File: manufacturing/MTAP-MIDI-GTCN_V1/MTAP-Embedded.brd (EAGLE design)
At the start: 160 x 100 mm, 32 parts, among them IC1 ESP32-WROOM-32D, IC2 AMS1117-3.3, X1 USB4140-GF-0230-C

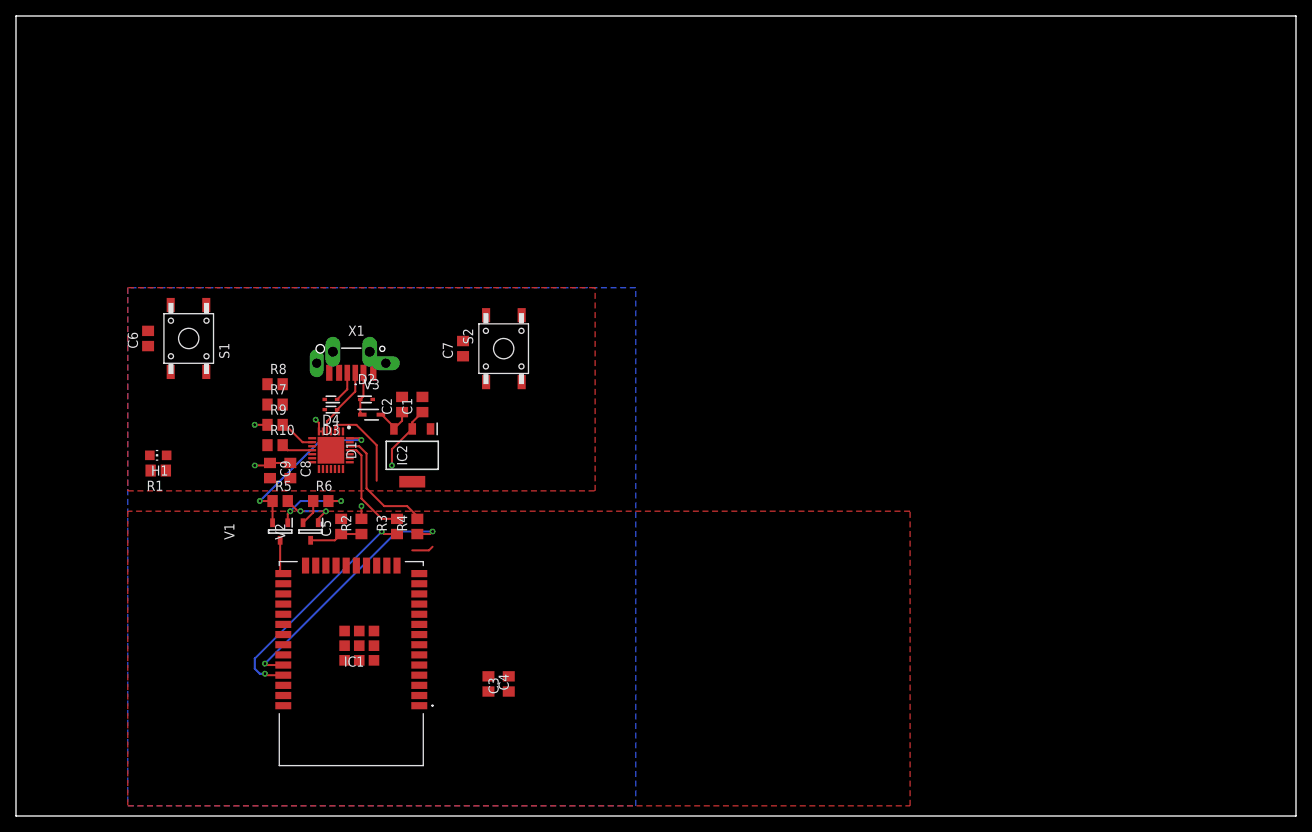
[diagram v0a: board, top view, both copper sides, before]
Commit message: upd Embedded
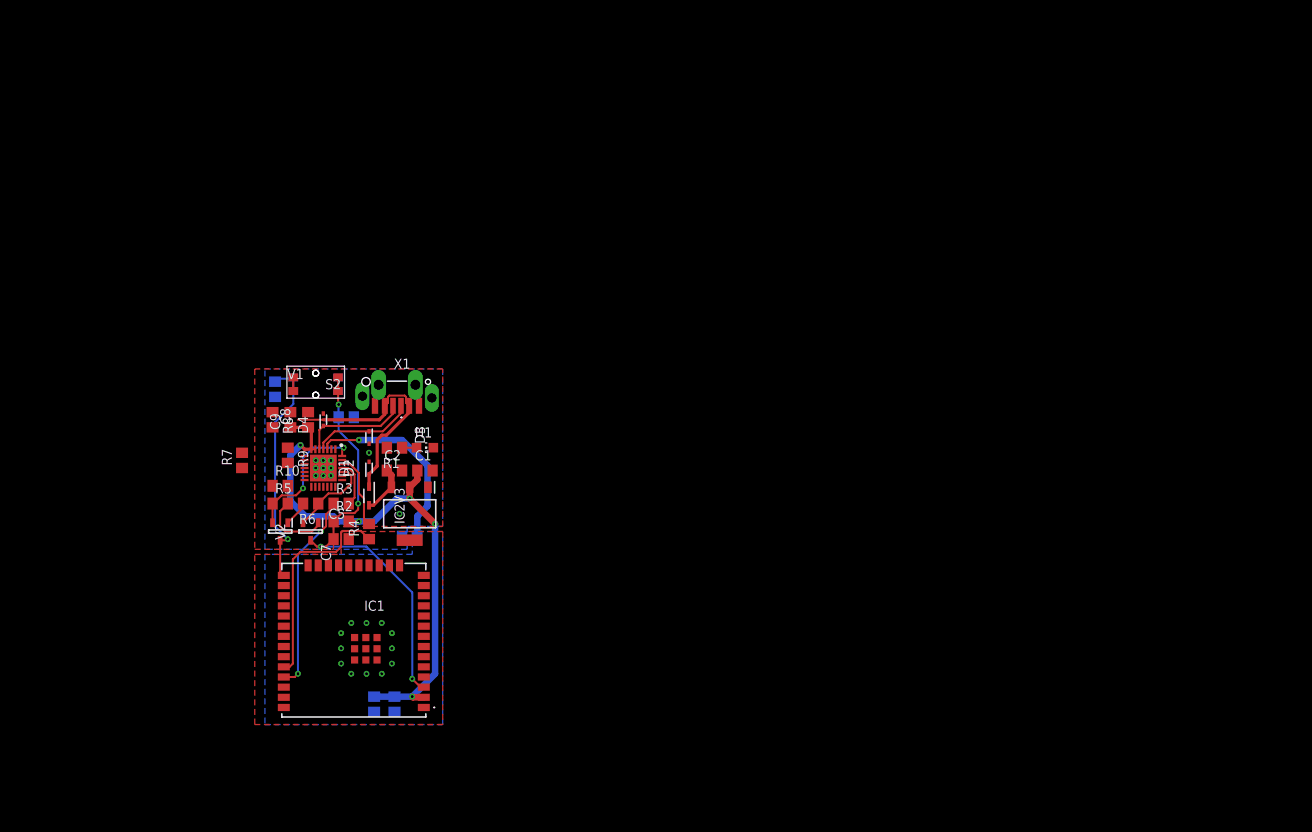
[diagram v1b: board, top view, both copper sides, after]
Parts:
- added R11: 0R, rcl_GruS:R0805
- IC1: value ESP32-WROOM-32D -> ESP32-WROOM-32UE-N8; device modul_GruS:ESP32WROOM32D4MBPS -> modul_GruS:ESP32WROOM32UEN8
- R7: value (none) -> 47k5
- R8: value (none) -> 22k1
- S1, S2: device switch_GruS:STS6X -> switch_GruS:WE_436331045822
- moved H1 33.4 mm to (51.1, 46.0), turned to 270 degrees
- moved R1 29.7 mm to (47.3, 46.0)
- moved S2 23.9 mm to (37.5, 54.0), turned to 180 degrees
- moved C6 17.1 mm to (32.4, 53.3), flipped to the bottom, turned to 270 degrees
- moved C3 17.0 mm to (44.8, 14.0), flipped to the bottom, turned to 270 degrees
- moved C7 16.9 mm to (41.3, 49.8), flipped to the bottom, turned to 180 degrees
- moved S1 16.9 mm to (37.5, 54.0), flipped to the bottom, turned to 180 degrees
- moved C4 12.0 mm to (47.3, 14.0), flipped to the bottom
- moved V3 10.2 mm to (44.1, 40.0), turned to 270 degrees
- moved D2 8.58 mm to (44.1, 43.5), turned to 90 degrees
- moved C2 8.31 mm to (47.3, 43.2), turned to 0 degrees
- moved C1 8.26 mm to (51.1, 43.2), turned to 0 degrees
- moved R7 8.11 mm to (28.3, 44.5), turned to 90 degrees
- moved R3 7.55 mm to (40.6, 39.1), turned to 0 degrees
- moved IC2 7.31 mm to (49.2, 37.8)
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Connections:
- net GND: now also R11.2
- net PGND: now also R11.1
- net USB_DN: now also D4.1, X1.B5; no longer D3.1, X1.A5
- net USB_DP: now also D3.1, X1.A5; no longer D4.1, X1.B5
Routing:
- net +3V3: track 18.1 -> 70.8 mm
- net EN: track 6.68 -> 54.0 mm, vias 0 -> 4
- net GPIO0: track 4.32 -> 29.8 mm, vias 0 -> 1
- net VBUS: track 5.50 -> 29.7 mm
- net GND: track 14.1 -> 24.1 mm, vias 0 -> 13
- net USB_DP: track 3.85 -> 13.0 mm
- net RTS: track 3.24 -> 10.6 mm
- net N$16: track 10.0 -> 3.18 mm, vias 2 -> 0
- net RXD: track 12.6 -> 5.84 mm
- net TXD: track 14.9 -> 9.44 mm
- net RXD0: track 32.2 -> 26.8 mm, vias 2 -> 0
- net USB_DN: track 8.80 -> 13.6 mm
- net TXD0: track 29.7 -> 25.0 mm
- net N$4: track 4.59 -> 0.00 mm
- net DTR: track 21.7 -> 17.5 mm
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- added copper zone on layer 16, net GND
- added copper zone on layer 16, net PGND
- removed copper zone on layer 16, net +3V3
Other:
- board outline removed

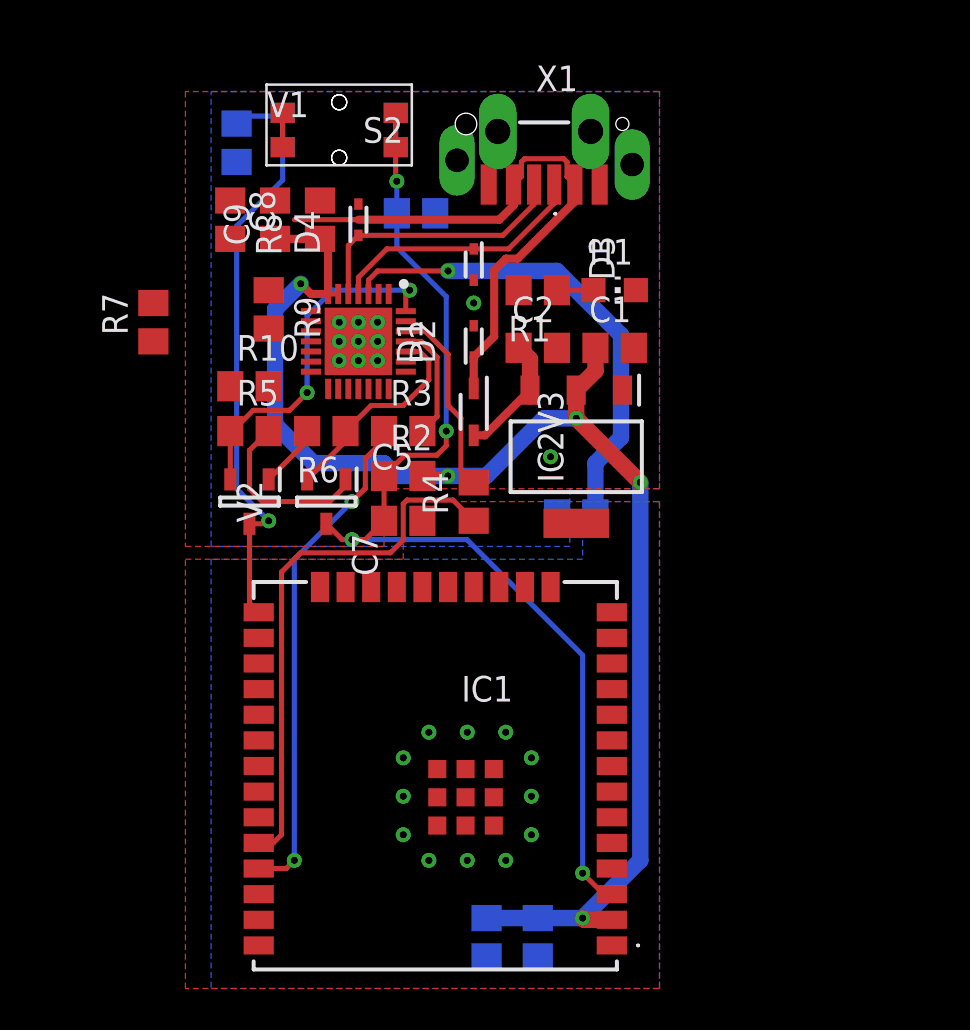
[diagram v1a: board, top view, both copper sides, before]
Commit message: upd embedded schematic
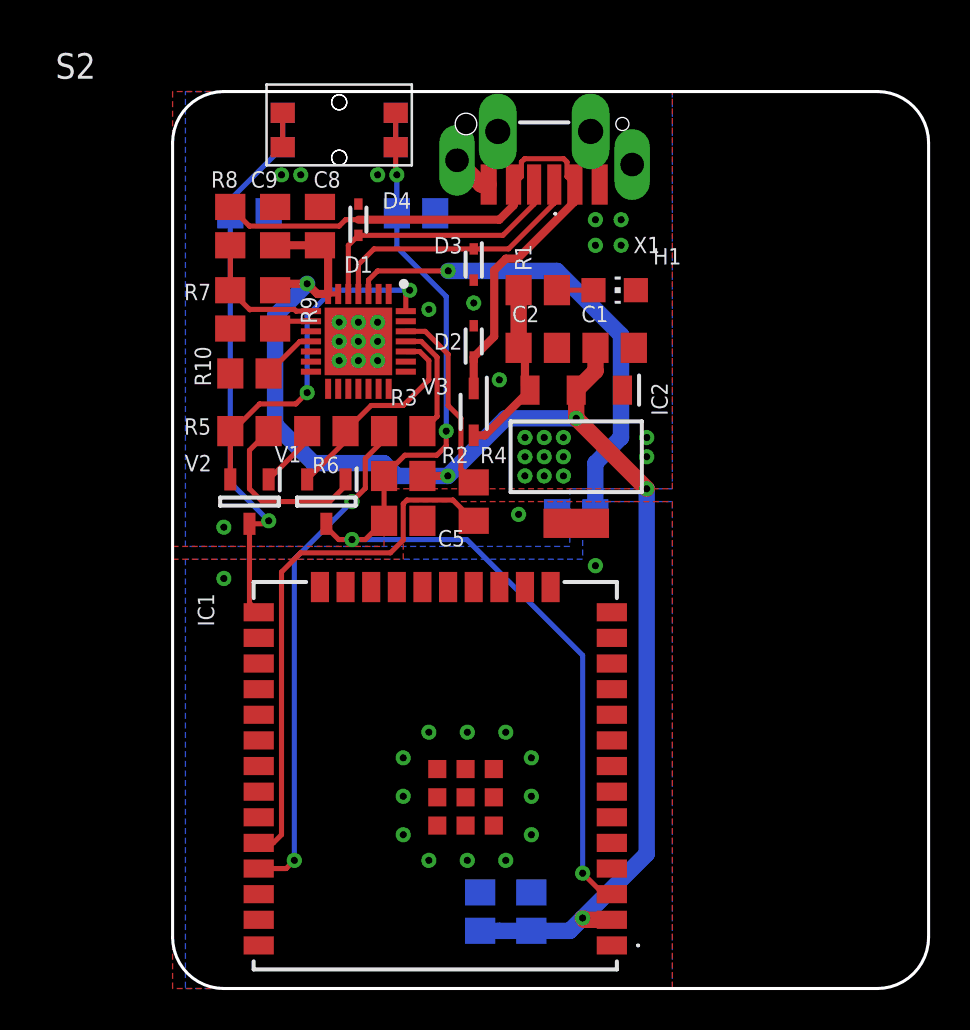
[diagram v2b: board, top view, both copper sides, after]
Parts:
- moved R7 3.86 mm to (32.1, 45.1)
- moved C6 3.55 mm to (33.0, 49.8), turned to 180 degrees
- moved C3 1.31 mm to (44.5, 15.2), turned to 90 degrees
- moved C4 1.31 mm to (47.0, 15.2), turned to 90 degrees
- moved R10 0.63 mm to (33.0, 41.9)
- moved C8 0.32 mm to (36.5, 49.2)
- moved C9 0.32 mm to (34.3, 49.2)
- moved R8 0.32 mm to (32.1, 49.2)
- moved R9 0.32 mm to (34.3, 45.1)
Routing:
- net N$2: track 0.00 -> 6.67 mm
- net VBUS: track 29.7 -> 33.4 mm
- net N$3: track 0.00 -> 2.78 mm
- net +5V: track 6.37 -> 8.91 mm
- net GPIO0: track 29.8 -> 27.7 mm
- net PGND: track 3.40 -> 5.40 mm, vias 11 -> 32
- net N$4: track 0.00 -> 1.93 mm
- net +3V3: track 70.8 -> 72.6 mm
- net GND: vias 13 -> 15
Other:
- board outline added: 37.5 x 44.5 mm
